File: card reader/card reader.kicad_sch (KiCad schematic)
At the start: 0 parts

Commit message: pdf
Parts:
- added A1: Arduino_Nano_v3.x, Module:Arduino_Nano, symbol MCU_Module:Arduino_Nano_v3.x
- added Q7: 2N7000, Package_TO_SOT_THT:TO-92_Inline, symbol Transistor_FET:2N7000
- added R1, R2, R26, R27, R3: 10k, symbol Device:R
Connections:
- new net: R2.2, R3.1
- new net +3.3V: Q7.2 (G), R26.1
- new net +5V: R27.1
- new net GND: R3.2
- new net RX_ARDUINO: Q7.3 (D), R27.2
- new net RX_RFID: R1.2, R2.1
- new net TX_ARDUINO: R1.1
- new net TX_RFID: Q7.1 (S), R26.2
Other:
- note added: "Adaptamos la tensión de 5 V a ~3.3 V (Arduino -> RFID reader)"
- note added: "Definir si se usa SPI o serial por soft. Seguramente si es spi se necesitan 3/4 conversores, si es serial solo 1 activo 1 pasivo. si es I2C idem serial"
- note added: "Esto es SPI seguro, al parecer es hard-wired"
- note added: "Subimos la tensión de 3.3 V a 5 V (RFID reader -> Arduino)"
- note added: "https://circuitdigest.com/microcontroller-projects/interfacing-rfid-reader-module-with-arduino"

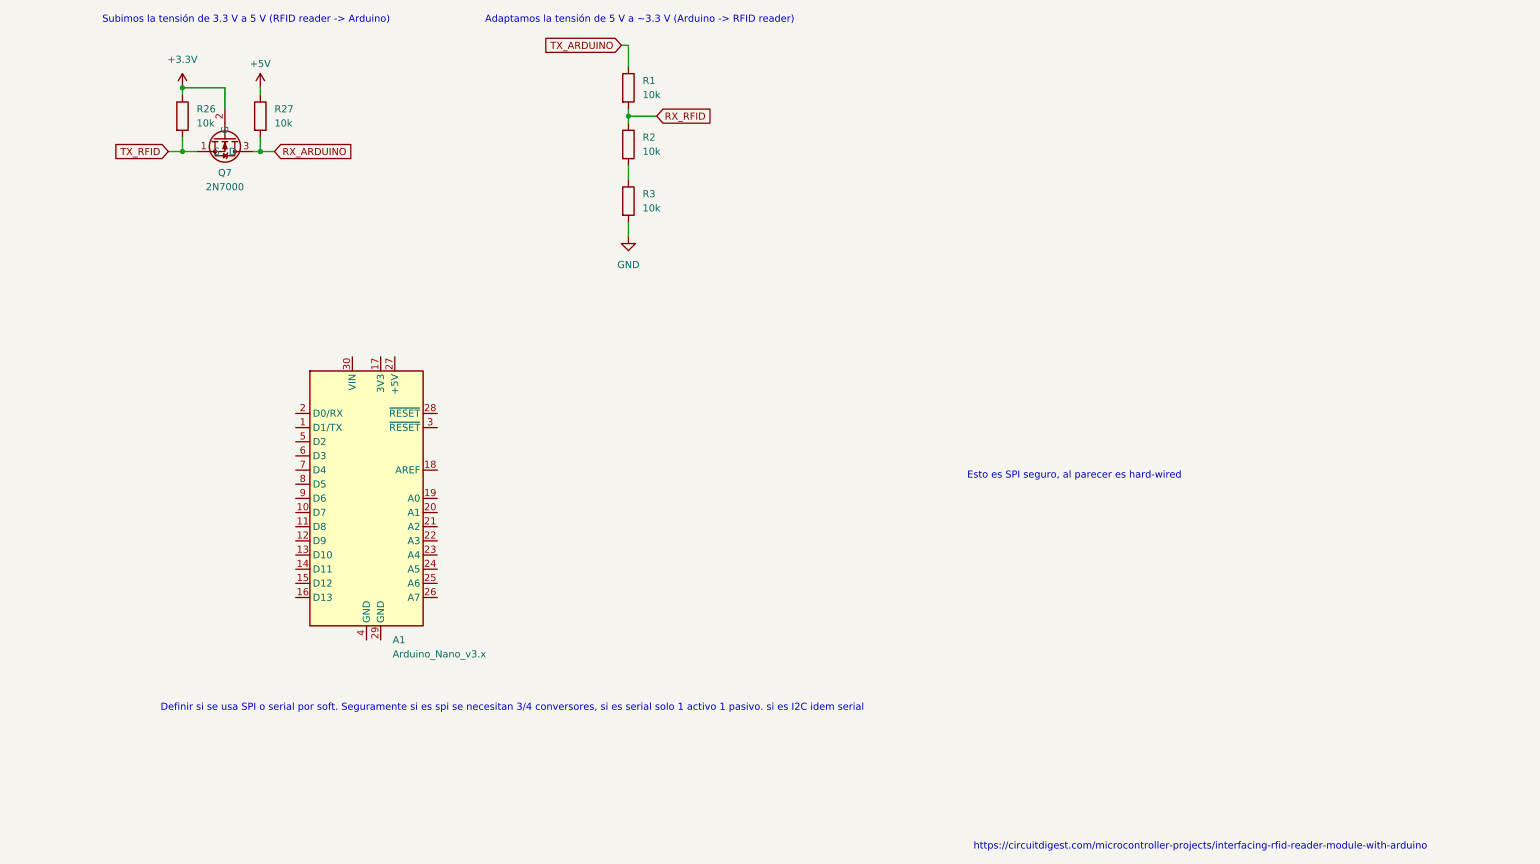
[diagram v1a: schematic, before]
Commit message: lolin module
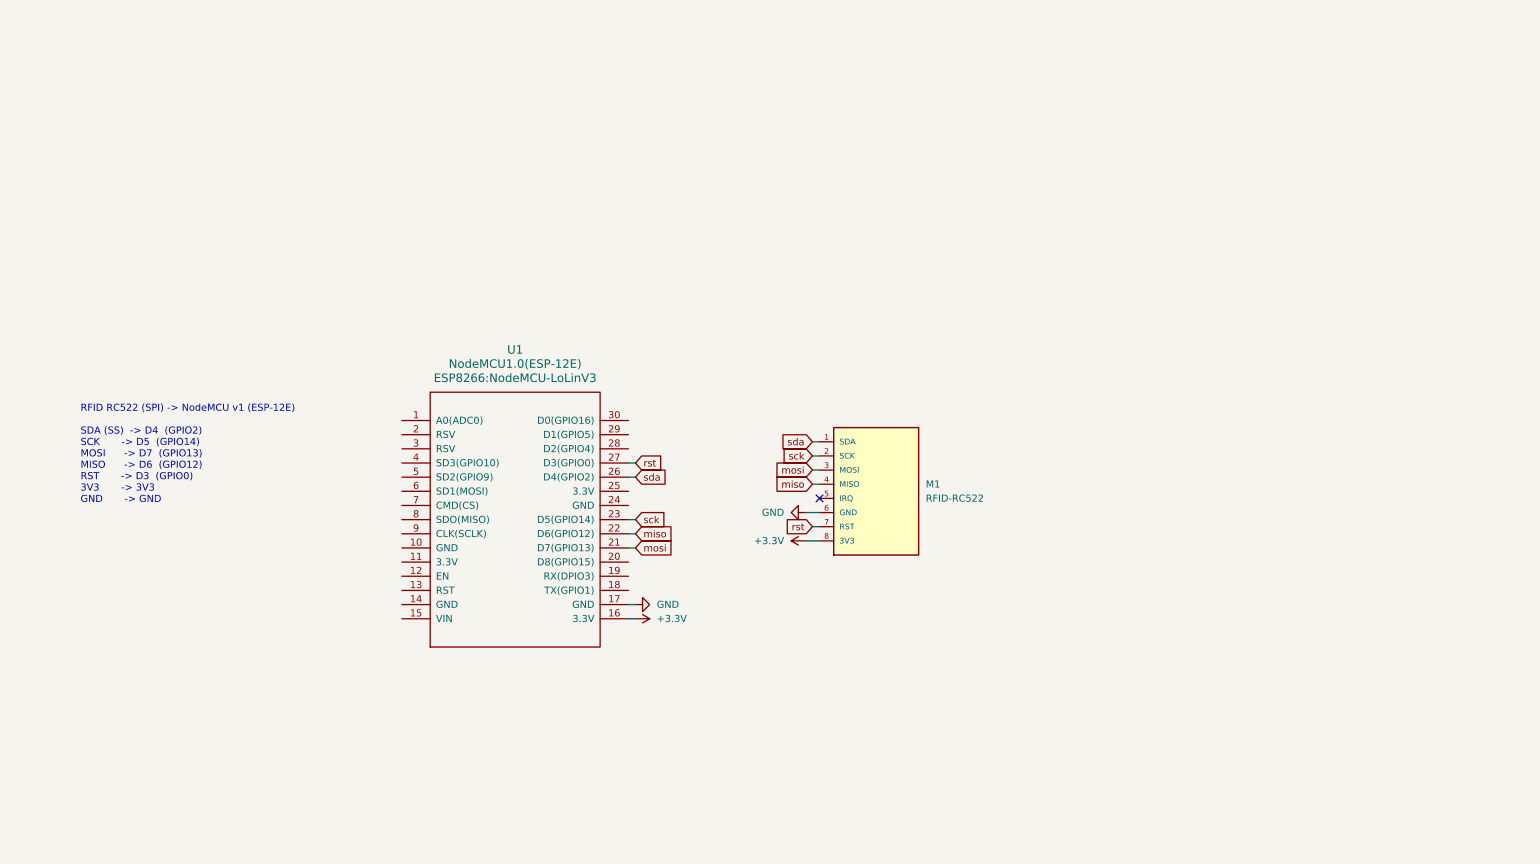
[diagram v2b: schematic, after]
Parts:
- removed A1: Arduino_Nano_v3.x, Module:Arduino_Nano, symbol MCU_Module:Arduino_Nano_v3.x
- removed Q7: 2N7000, Package_TO_SOT_THT:TO-92_Inline, symbol Transistor_FET:2N7000
- removed R1, R2, R26, R27, R3: 10k, symbol Device:R
- added M1: RFID-RC522, RFID-RC522:RFID-RC522, symbol RFID-RC522:RFID-RC522
- added U1: NodeMCU1.0(ESP-12E), ESP8266:NodeMCU-LoLinV3, symbol ESP8266:NodeMCU1.0(ESP-12E)
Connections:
- net +3.3V: now also M1.8 (3V3), U1.16 (3.3V)
- net GND: now also M1.6 (GND), U1.17 (GND)
- new net miso: M1.4 (MISO), U1.22 (D6(GPIO12))
- new net mosi: M1.3 (MOSI), U1.21 (D7(GPIO13))
- new net rst: M1.7 (RST), U1.27 (D3(GPIO0))
- new net sck: M1.2 (SCK), U1.23 (D5(GPIO14))
- new net sda: M1.1 (SDA), U1.26 (D4(GPIO2))
- no-connect marks 0 -> 1
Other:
- note added: "RFID RC522 (SPI) -> NodeMCU v1 (ESP-12E) SDA (SS) -> D4 (GPIO2) SCK -> D5 (GPIO14) MOSI -> D7 (GPIO13) MISO -> D6 (GPIO12) RST -> D3 (GPIO0) 3V3 -> 3V3 GND -> GND"
- note removed: "Adaptamos la tensión de 5 V a ~3.3 V (Arduino -> RFID reader)"
- note removed: "Definir si se usa SPI o serial por soft. Seguramente si es spi se necesitan 3/4 conversores, si es serial solo 1 activo 1 pasivo. si es I2C idem serial"
- note removed: "Esto es SPI seguro, al parecer es hard-wired"
- note removed: "Subimos la tensión de 3.3 V a 5 V (RFID reader -> Arduino)"
- note removed: "https://circuitdigest.com/microcontroller-projects/interfacing-rfid-reader-module-with-arduino"
